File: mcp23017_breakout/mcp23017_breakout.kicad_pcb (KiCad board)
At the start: 2 copper layers, 16 x 29 mm, 10 parts, among them U1 address_sel, U2 address_sel, U3 address_sel, U4 MCP23017

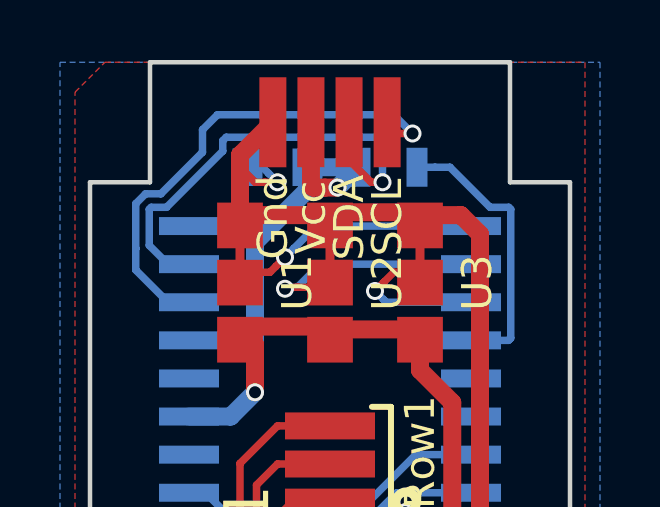
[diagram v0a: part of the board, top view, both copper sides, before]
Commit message: bugfixing
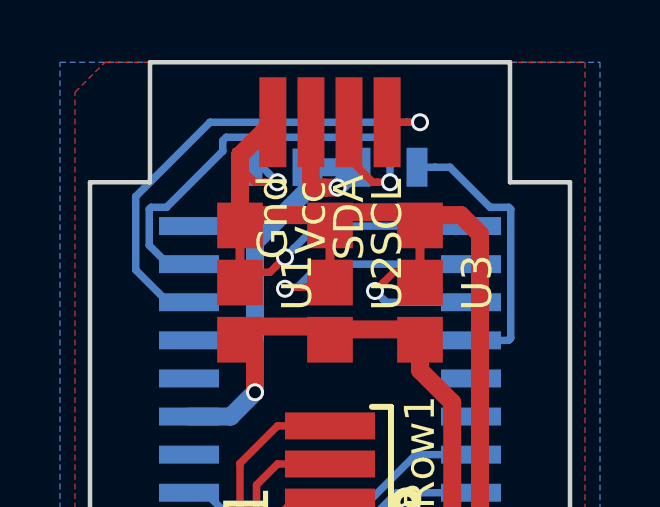
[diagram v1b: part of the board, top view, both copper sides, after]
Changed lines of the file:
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@@
     (links 38)
     (no_connects 1)
-    (area 41.924999 44.924999 58.075001 74.075001)
+    (area 40.974999 38.3 72.135715 89.000001)
     (thickness 1.6)
     (drawings 27)
-    (tracks 267)
+    (tracks 263)
     (zones 0)
     (modules 10)
@@
     (uvia_drill 0.1)
   )
-  (module myComponents:solderPads_4_Grove_I2C (layer F.Cu)
-    (at 50 47 180)
-    (fp_text reference I2C1 (at 0.635 2.54 180) (layer F.SilkS) hide
-      (effects (font (size 1 1) (thickness 0.15)))
-    )
-    (fp_text value CONN_01X04 (at 0.635 2.54 180) (layer F.Fab)
-      (effects (font (size 1 1) (thickness 0.15)))
-    )
-    (fp_text user SDA (at -0.635 -3.175 270) (layer F.SilkS)
-      (effects (font (size 1 1) (thickness 0.15)))
-    )
-    (fp_text user SCL (at -1.905 -3.175 270) (layer F.SilkS)
-      (effects (font (size 1 1) (thickness 0.15)))
-    )
-    (fp_text user Gnd (at 1.905 -3.175 270) (layer F.SilkS)
-      (effects (font (size 1 1) (thickness 0.15)))
-    )
-    (fp_text user Vcc (at 0.635 -3.175 270) (layer F.SilkS)
-      (effects (font (size 1 1) (thickness 0.15)))
-    )
-    (pad 1 smd rect (at -1.905 0 180) (size 0.9 3) (layers F.Cu F.Paste F.Mask)
-      (net 9 /SCL))
-    (pad 2 smd rect (at -0.635 0 180) (size 0.9 3) (layers F.Cu F.Paste F.Mask)
-      (net 10 /SDA))
-    (pad 3 smd rect (at 0.635 0 180) (size 0.9 3) (layers F.Cu F.Paste F.Mask)
-      (net 7 +5V))
-    (pad 4 smd rect (at 1.905 0 180) (size 0.9 3) (layers F.Cu F.Paste F.Mask)
-      (net 8 GND))
-  )
   (module Resistors_SMD:R_0805 (layer B.Cu)
     (at 51.95 48.5 180)
@@
       (rotate (xyz 0 0 0))
     )
+  )
+  (module myComponents:solderPads_4_Grove_I2C (layer F.Cu)
+    (at 50 47 180)
+    (fp_text reference I2C1 (at 0.635 2.54 180) (layer F.SilkS) hide
+      (effects (font (size 1 1) (thickness 0.15)))
+    )
+    (fp_text value CONN_01X04 (at 0.635 2.54 180) (layer F.Fab)
+      (effects (font (size 1 1) (thickness 0.15)))
+    )
+    (fp_text user SDA (at -0.635 -3.175 270) (layer F.SilkS)
+      (effects (font (size 1 1) (thickness 0.15)))
+    )
+    (fp_text user SCL (at -1.905 -3.175 270) (layer F.SilkS)
+      (effects (font (size 1 1) (thickness 0.15)))
+    )
+    (fp_text user Gnd (at 1.905 -3.175 270) (layer F.SilkS)
+      (effects (font (size 1 1) (thickness 0.15)))
+    )
+    (fp_text user Vcc (at 0.635 -3.175 270) (layer F.SilkS)
+      (effects (font (size 1 1) (thickness 0.15)))
+    )
+    (pad 1 smd rect (at -1.905 0 180) (size 0.9 3) (layers F.Cu F.Paste F.Mask)
+      (net 9 /SCL))
+    (pad 2 smd rect (at -0.635 0 180) (size 0.9 3) (layers F.Cu F.Paste F.Mask)
+      (net 10 /SDA))
+    (pad 3 smd rect (at 0.635 0 180) (size 0.9 3) (layers F.Cu F.Paste F.Mask)
+      (net 7 +5V))
+    (pad 4 smd rect (at 1.905 0 180) (size 0.9 3) (layers F.Cu F.Paste F.Mask)
+      (net 8 GND))
   )
   (module myComponents:solderPads_6 (layer F.Cu)
@@
   (segment (start 49.905 50.095) (end 50 50) (width 0.6) (layer F.Cu) (net 8))
   (segment (start 47.1 48.5) (end 47.1 48.2) (width 0.25) (layer B.Cu) (net 8))
+  (segment (start 52.575736 47) (end 53 47) (width 0.25) (layer B.Cu) (net 9))
+  (segment (start 46 47) (end 52.575736 47) (width 0.25) (layer B.Cu) (net 9))
+  (segment (start 44.6 53) (end 43.52499 51.92499) (width 0.25) (layer B.Cu) (net 9))
+  (segment (start 43.52499 49.47501) (end 46 47) (width 0.25) (layer B.Cu) (net 9))
   (segment (start 45.3 53) (end 44.6 53) (width 0.25) (layer B.Cu) (net 9))
-  (segment (start 43.853599 49.384988) (end 44.365012 49.384988) (width 0.25) (layer B.Cu) (net 9))
-  (segment (start 44.6 53) (end 43.52499 51.92499) (width 0.25) (layer B.Cu) (net 9))
-  (segment (start 43.524988 51.206401) (end 43.524988 49.713599) (width 0.25) (layer B.Cu) (net 9))
-  (segment (start 45.75 48) (end 45.75 47.25) (width 0.25) (layer B.Cu) (net 9))
-  (segment (start 52.125002 46.75) (end 52.75 47.374998) (width 0.25) (layer B.Cu) (net 9))
-  (segment (start 43.52499 51.92499) (end 43.52499 51.206403) (width 0.25) (layer B.Cu) (net 9))
-  (segment (start 43.52499 51.206403) (end 43.524988 51.206401) (width 0.25) (layer B.Cu) (net 9))
-  (segment (start 43.524988 49.713599) (end 43.853599 49.384988) (width 0.25) (layer B.Cu) (net 9))
-  (segment (start 45.75 47.25) (end 46.25 46.75) (width 0.25) (layer B.Cu) (net 9))
-  (segment (start 44.365012 49.384988) (end 45.75 48) (width 0.25) (layer B.Cu) (net 9))
-  (segment (start 46.25 46.75) (end 52.125002 46.75) (width 0.25) (layer B.Cu) (net 9))
-  (segment (start 52.75 47.374998) (end 52.279998 47.374998) (width 0.25) (layer F.Cu) (net 9))
-  (segment (start 52.279998 47.374998) (end 51.905 47) (width 0.25) (layer F.Cu) (net 9))
-  (via (at 52.75 47.374998) (size 0.6) (drill 0.4) (layers F.Cu B.Cu) (net 9))
-  (segment (start 51.75 49) (end 51.75 47.664998) (width 0.25) (layer B.Cu) (net 10))
-  (segment (start 51.75 47.664998) (end 51.585002 47.5) (width 0.25) (layer B.Cu) (net 10))
-  (segment (start 51.585002 47.5) (end 46.539998 47.5) (width 0.25) (layer B.Cu) (net 10))
-  (segment (start 46.539998 47.5) (end 46.424999 47.614999) (width 0.25) (layer B.Cu) (net 10))
-  (segment (start 44.551411 49.834999) (end 44.039999 49.834999) (width 0.25) (layer B.Cu) (net 10))
-  (segment (start 46.424999 47.614999) (end 46.424999 47.961411) (width 0.25) (layer B.Cu) (net 10))
-  (segment (start 46.424999 47.961411) (end 44.551411 49.834999) (width 0.25) (layer B.Cu) (net 10))
-  (segment (start 44.039999 49.834999) (end 43.974999 49.899999) (width 0.25) (layer B.Cu) (net 10))
-  (segment (start 43.974999 49.899999) (end 43.974999 51.104999) (width 0.25) (layer B.Cu) (net 10))
-  (segment (start 43.974999 51.104999) (end 44.6 51.73) (width 0.25) (layer B.Cu) (net 10))
-  (segment (start 44.6 51.73) (end 45.3 51.73) (width 0.25) (layer B.Cu) (net 10))
-  (segment (start 50.635 47) (end 50.635 48.265002) (width 0.25) (layer F.Cu) (net 10))
-  (segment (start 50.635 48.265002) (end 51.369998 49) (width 0.25) (layer F.Cu) (net 10))
-  (segment (start 51.369998 49) (end 51.75 49) (width 0.25) (layer F.Cu) (net 10))
-  (via (at 51.75 49) (size 0.6) (drill 0.4) (layers F.Cu B.Cu) (net 10))
+  (segment (start 51.905 47) (end 53 47) (width 0.25) (layer F.Cu) (net 9))
+  (segment (start 43.52499 51.92499) (end 43.52499 49.47501) (width 0.25) (layer B.Cu) (net 9))
+  (via (at 53 47) (size 0.6) (drill 0.4) (layers F.Cu B.Cu) (net 9))
+  (segment (start 52 49.000002) (end 52 47.915026) (width 0.25) (layer B.Cu) (net 10))
+  (segment (start 52 47.915026) (end 52.000014 47.915012) (width 0.25) (layer B.Cu) (net 10))
+  (segment (start 51.57575 49) (end 51.999998 49) (width 0.25) (layer F.Cu) (net 10))
+  (segment (start 51.999998 49) (end 52 49.000002) (width 0.25) (layer F.Cu) (net 10))
+  (via (at 52 49.000002) (size 0.6) (drill 0.4) (layers F.Cu B.Cu) (net 10))
+  (segment (start 46.424999 47.961411) (end 46.424999 47.614999) (width 0.25) (layer B.Cu) (net 10))
+  (segment (start 51.585002 47.5) (end 52.000014 47.915012) (width 0.25) (layer B.Cu) (net 10))
+  (segment (start 46.424999 47.614999) (end 46.539998 47.5) (width 0.25) (layer B.Cu) (net 10))
+  (segment (start 46.539998 47.5) (end 51.585002 47.5) (width 0.25) (layer B.Cu) (net 10))
+  (segment (start 44.551411 49.834999) (end 46.424999 47.961411) (width 0.25) (layer B.Cu) (net 10))
+  (segment (start 44.039999 49.834999) (end 44.551411 49.834999) (width 0.25) (layer B.Cu) (net 10))
+  (segment (start 43.974999 51.104999) (end 43.974999 49.899999) (width 0.25) (layer B.Cu) (net 10))
+  (segment (start 44.6 51.73) (end 43.974999 51.104999) (width 0.25) (layer B.Cu) (net 10))
+  (segment (start 50.635 48.209206) (end 51.425794 49) (width 0.25) (layer F.Cu) (net 10))
+  (segment (start 45.3 51.73) (end 44.6 51.73) (width 0.25) (layer B.Cu) (net 10))
+  (segment (start 43.974999 49.899999) (end 44.039999 49.834999) (width 0.25) (layer B.Cu) (net 10))
+  (segment (start 51.425794 49) (end 51.57575 49) (width 0.25) (layer F.Cu) (net 10))
+  (segment (start 50.635 47) (end 50.635 48.209206) (width 0.25) (layer F.Cu) (net 10))
   (segment (start 50.635 72.87) (end 49.182001 71.417001) (width 0.25) (layer B.Cu) (net 11))
   (segment (start 49.182001 71.417001) (end 48.843239 71.417001) (width 0.25) (layer B.Cu) (net 11))
